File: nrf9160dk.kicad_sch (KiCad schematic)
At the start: 3 parts, among them U1 NRF9160-DK

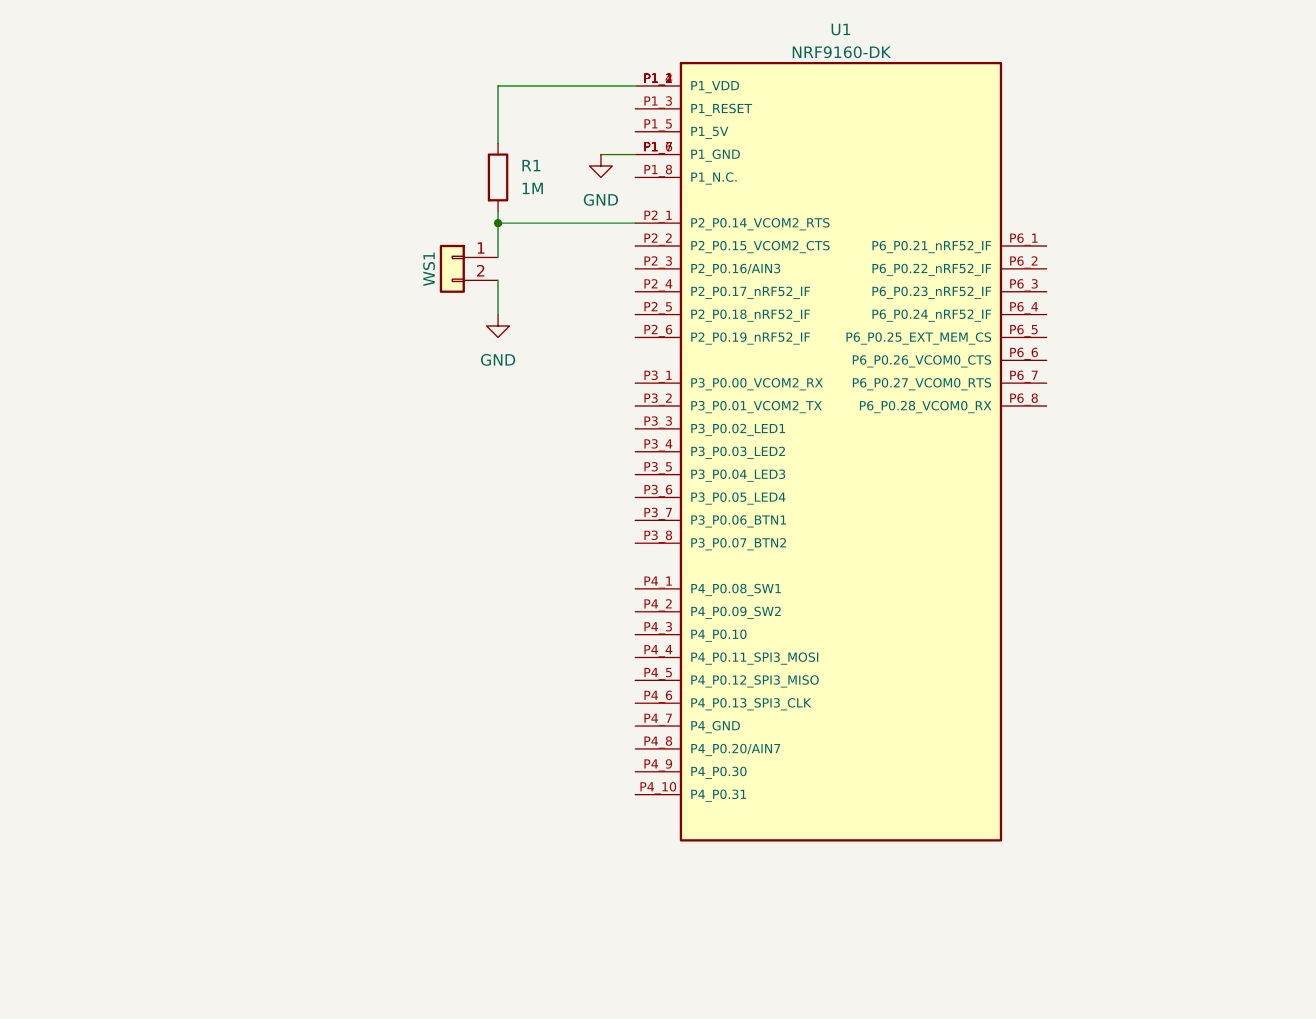
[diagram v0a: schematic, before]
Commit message: board v1.0
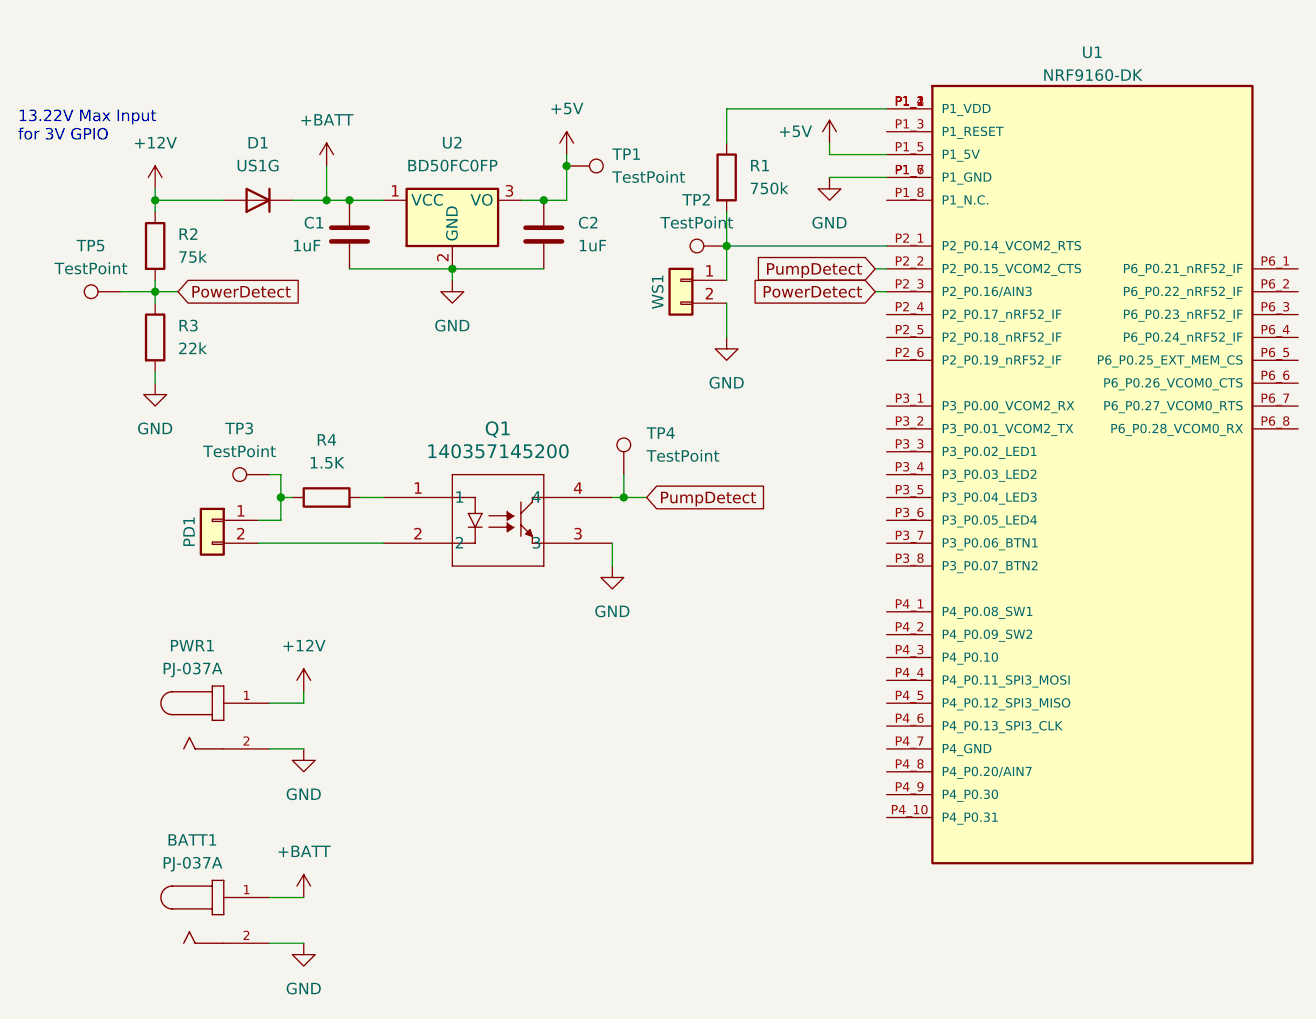
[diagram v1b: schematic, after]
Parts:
- added BATT1, PWR1: PJ-037A, PJ-037A:CUI_PJ-037A, symbol PJ-037A:PJ-037A
- added C1, C2: 1uF, Capacitor_SMD:C_0603_1608Metric_Pad1.08x0.95mm_HandSolder, symbol Device:C
- added D1: US1G, Diode_SMD:D_SMA, symbol Diode:US1G
- added PD1: Conn_01x02, Connector_PinHeader_2.54mm:PinHeader_1x02_P2.54mm_Vertical, symbol Connector_Generic:Conn_01x02
- added Q1: 140357145200, footprints:WL-OCPT_SOP4_WRE, symbol 2024-04-10_19-53-40:140357145200
- added R2: 75k, Resistor_SMD:R_0805_2012Metric_Pad1.20x1.40mm_HandSolder, symbol Device:R
- added R3: 22k, Resistor_SMD:R_0805_2012Metric_Pad1.20x1.40mm_HandSolder, symbol Device:R
- added R4: 1.5K, Resistor_SMD:R_0805_2012Metric_Pad1.20x1.40mm_HandSolder, symbol Device:R
- added TP1, TP2, TP3, TP4, TP5: TestPoint, TestPoint:TestPoint_Pad_D1.0mm, symbol Connector:TestPoint
- added U2: BD50FC0FP, Package_TO_SOT_SMD:TO-252-2, symbol Regulator_Linear:BD50FC0FP
- R1: value 1M -> 750k
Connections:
- net GND: now also BATT1.2, C1.2, C2.2, PWR1.2, Q1.3, R3.2, U2.2 (GND)
- net +5V: now reaches U1.P1_5 (P1_5V)
- net +5V: now also C2.1, TP1.1, U2.3 (VO)
- net at R1.2, U1.P2_1 (P2_P0.14_VCOM2_RTS), WS1.1 (Pin_1): now also TP2.1
- net PumpDetect: now reaches U1.P2_2 (P2_P0.15_VCOM2_CTS)
- net PumpDetect: now also Q1.4, TP4.1
- net PowerDetect: now reaches U1.P2_3 (P2_P0.16/AIN3)
- net PowerDetect: now also R2.2, R3.1, TP5.1
- new net: PD1.1 (Pin_1), R4.1, TP3.1
- new net: PD1.2 (Pin_2), Q1.2
- new net: Q1.1, R4.2
- new net +12V: D1.2 (A), PWR1.1, R2.1
- new net +BATT: BATT1.1, C1.1, D1.1 (K), U2.1 (VCC)
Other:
- note added: "13.22V Max Input for 3V GPIO"
- moved on the sheet: R1, U1, WS1
